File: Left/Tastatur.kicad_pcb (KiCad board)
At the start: 2 copper layers, 125.5 x 85.1 mm, 145 parts, among them J102 Conn_01x04_Pin, J103 XT60PW-M, Q101 SI2301CDS-T1-GE3, Q102 SI2301CDS-T1-GE3, Q103 SI2301CDS-T1-GE3, Q104 SI2301CDS-T1-GE3, Q105 SI2301CDS-T1-GE3, Q106 2N7002HW, Q107 SI2301CDS-T1-GE3, SW201 SW_Push, SW202 SW_Push, SW203 SW_Push, SW204 SW_Push, SW205 SW_Push, SW206 SW_Push, SW207 SW_Push, SW208 SW_Push, SW209 SW_Push, SW210 SW_Push, SW211 SW_Push, SW212 SW_Push, SW213 SW_Push, SW214 SW_Push, SW215 SW_Push, SW216 SW_Push, SW217 SW_Push, SW218 SW_Push, SW219 SW_Push, SW221 MK-12C02-G020, U101 USBLC6-2SC6, U102 CH592F, U103 AP2112K-3.3, U104 MT3608, U105 TP4056-42-ESOP8, U106 CD4052B, U107 LM393, Y101 32MHz

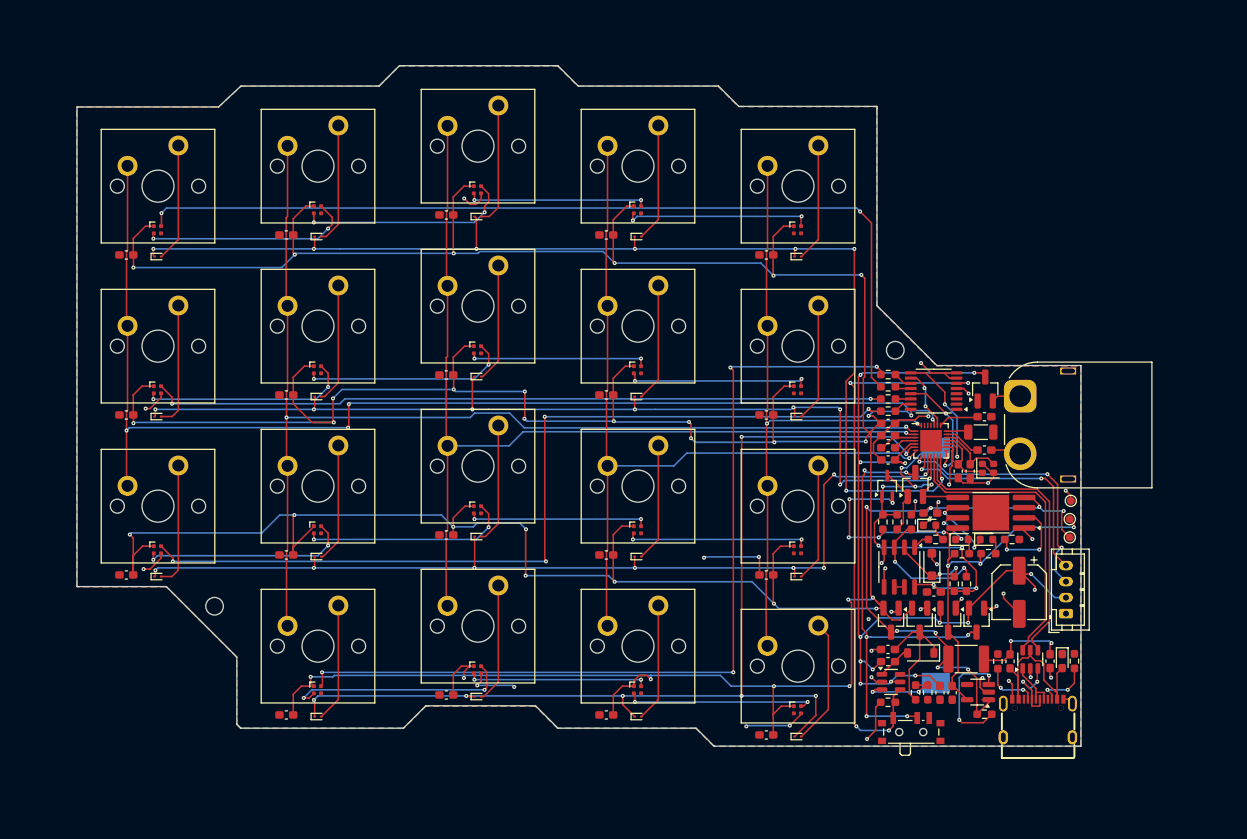
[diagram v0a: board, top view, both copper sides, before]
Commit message: update
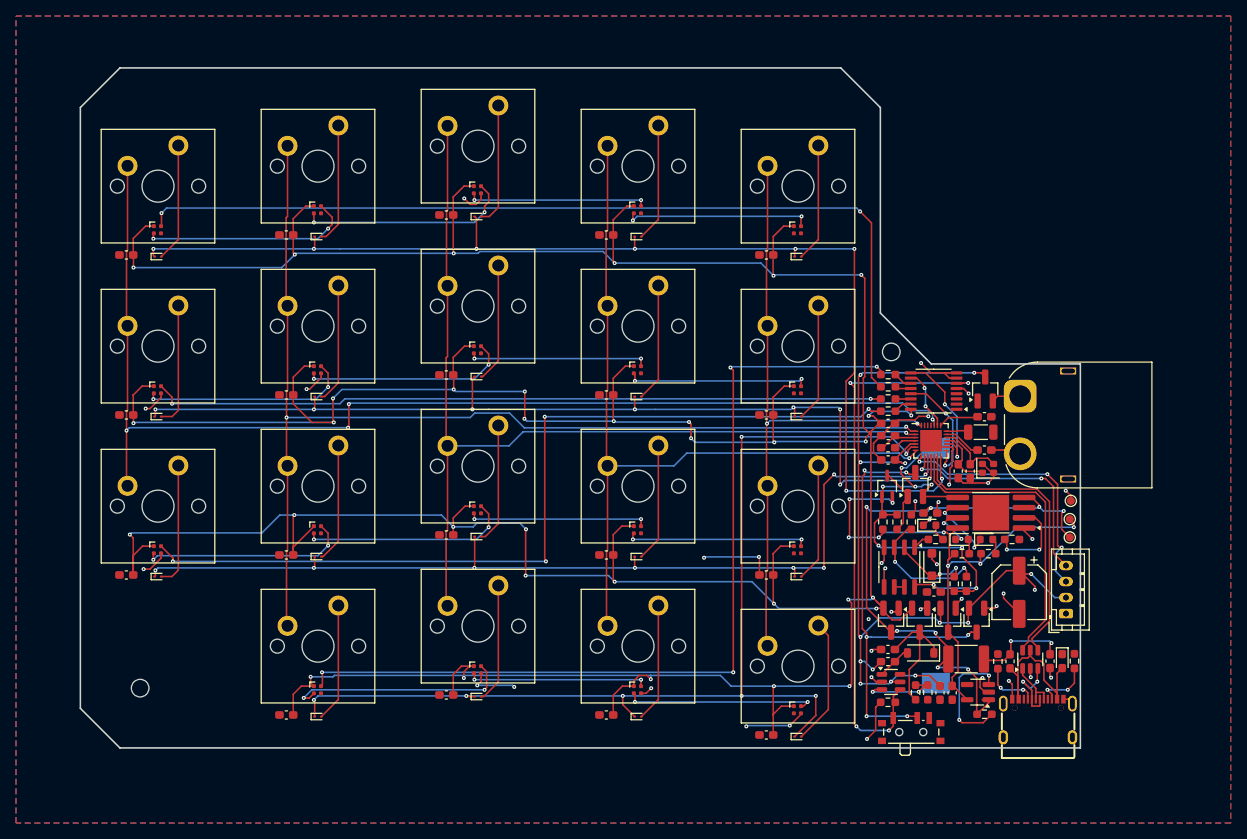
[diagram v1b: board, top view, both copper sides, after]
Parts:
- moved H201 13.8 mm to (80.9, 132.4)
- moved H202 0.55 mm to (174.8, 90.4)
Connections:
- AE101 pad 2: GNDS -> GND
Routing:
- net GND: track 111.4 -> 115.9 mm, vias 34 -> 36
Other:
- board size 125.5 x 85.1 mm -> 125 x 85 mm
